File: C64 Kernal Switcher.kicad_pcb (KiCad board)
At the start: 2 copper layers, 8 parts, among them J1 LED, J2 Signals, U1 2364, U2 28C256

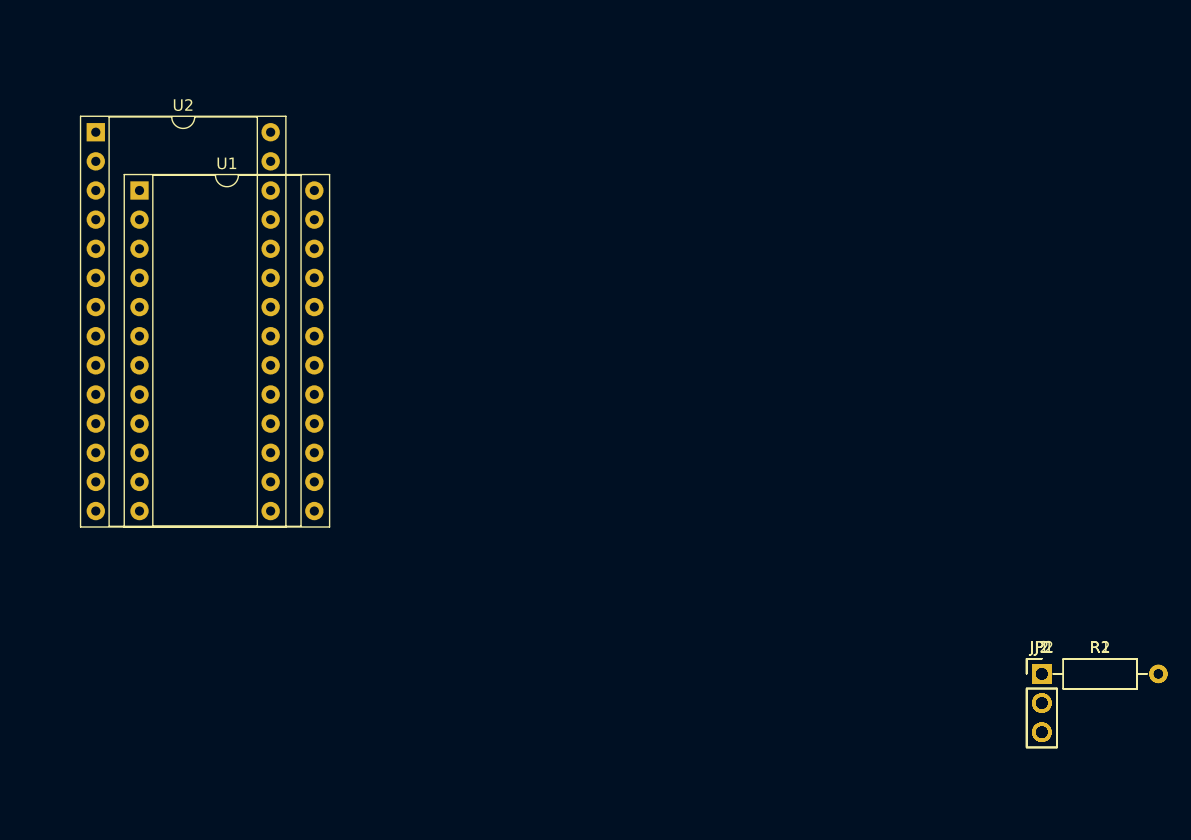
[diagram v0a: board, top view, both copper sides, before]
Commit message: PCB layed out, need measuring
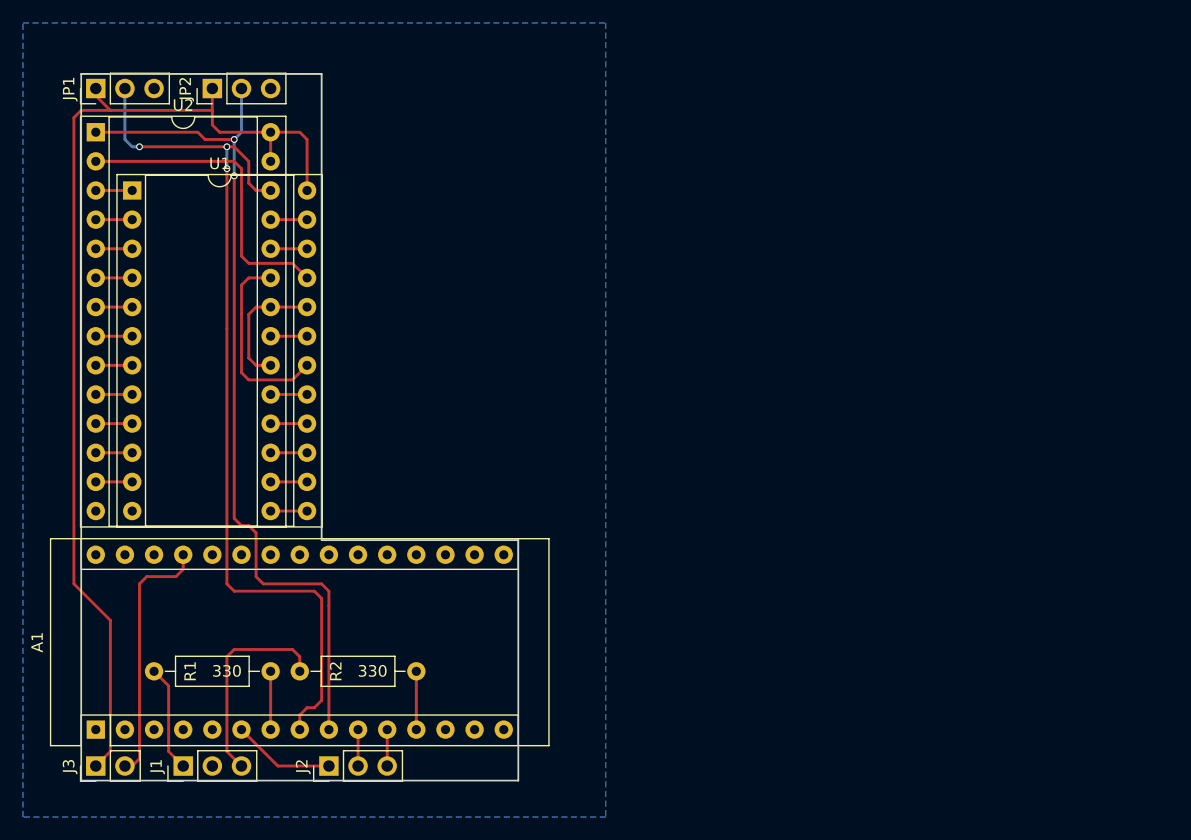
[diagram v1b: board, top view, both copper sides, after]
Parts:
- added A1: Arduino_Nano_v3.x, Modules:Arduino_Nano, F.Cu at (66.0, 109.9)
- added J3: Power, Pin_Headers:Pin_Header_Straight_1x02_Pitch2.54mm, F.Cu at (66.0, 113.0)
- moved JP1 97.0 mm to (66.0, 54.0), turned to 90 degrees
- moved JP2 88.5 mm to (76.2, 54.0), turned to 90 degrees
- moved R1 77.4 mm to (71.1, 104.8)
- moved J1 75.3 mm to (73.7, 113.0), turned to 90 degrees
- moved R2 64.7 mm to (83.8, 104.8)
- moved J2 62.7 mm to (86.4, 113.0), turned to 90 degrees
- moved U1 0.63 mm to (69.2, 62.9)
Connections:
- J2 pad 1: (no net) -> ESXROM
- J2 pad 2: (no net) -> RESET
- J2 pad 3: (no net) -> RESTORE
- R1 pad 2: (no net) -> LED1
- R2 pad 2: (no net) -> LED2
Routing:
- net VCC: track 0.00 -> 92.1 mm
- net A13: track 0.00 -> 79.6 mm, vias 0 -> 3
- net A14: track 0.00 -> 75.2 mm, vias 0 -> 2
- net /A12: track 0.00 -> 27.1 mm
- net Net-(A1-Pad27): track 0.00 -> 22.4 mm
- net Net-(J1-Pad3): track 0.00 -> 18.2 mm
- net /A11: track 0.00 -> 16.9 mm
- net /CS: track 0.00 -> 11.3 mm
- net Net-(J1-Pad1): track 0.00 -> 9.31 mm
- net ESXROM: track 0.00 -> 8.94 mm
- net LED2: track 0.00 -> 5.08 mm
- net LED1: track 0.00 -> 5.08 mm
- net RESTORE: track 0.00 -> 3.81 mm
- net RESET: track 0.00 -> 3.81 mm
- net /D7: track 0.00 -> 3.17 mm
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- added copper zone on B.Cu, net GND
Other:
- board outline added: 38.1 x 61.6 mm

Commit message: Layout redone
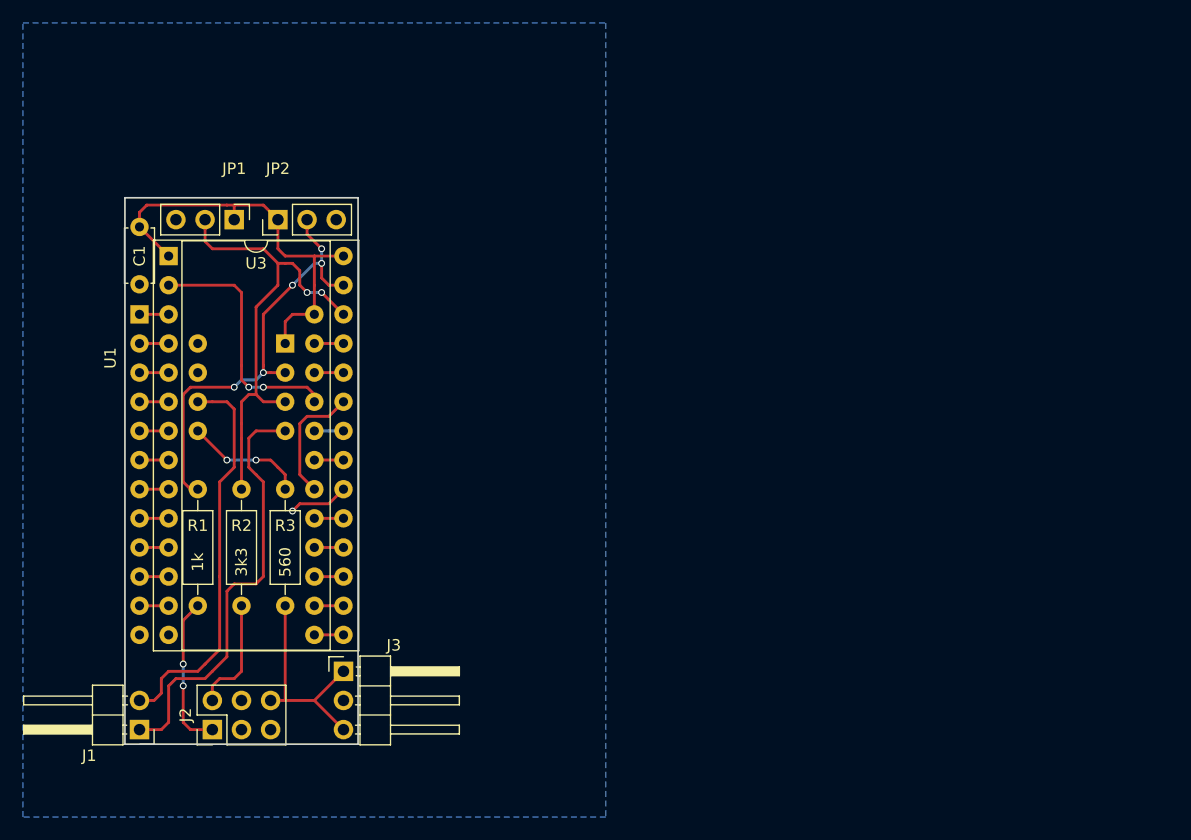
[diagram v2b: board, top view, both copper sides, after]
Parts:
- removed A1: Arduino_Nano_v3.x, Modules:Arduino_Nano
- added C1: 100nF, Capacitors_THT:C_Disc_D4.7mm_W2.5mm_P5.00mm, F.Cu at (69.8, 66.0)
- added R3: 560, Resistors_THT:R_Axial_DIN0207_L6.3mm_D2.5mm_P10.16mm_Horizontal, F.Cu at (82.5, 99.1)
- added U3: 27C256, Housings_DIP:DIP-28_W15.24mm_Socket, F.Cu at (72.4, 68.6)
- J1: value LED -> Signals; footprint Pin_Headers:Pin_Header_Straight_1x03_Pitch2.54mm -> Pin_Headers:Pin_Header_Angled_1x02_Pitch2.54mm
- J2: value Signals -> RGB; footprint Pin_Headers:Pin_Header_Straight_1x03_Pitch2.54mm -> Pin_Headers:Pin_Header_Straight_2x03_Pitch2.54mm
- J3: value Power -> LED; footprint Pin_Headers:Pin_Header_Straight_1x02_Pitch2.54mm -> Pin_Headers:Pin_Header_Angled_1x03_Pitch2.54mm
- R1: value 330 -> 1k
- R2: value 330 -> 3k3
- U1: footprint Housings_DIP:DIP-24_W15.24mm_Socket -> 2364:DIP-24_W15.24mm_Socket
- U2: value 28C256 -> PIC12F629-I/MS; footprint Housings_DIP:DIP-28_W15.24mm_Socket -> Housings_DIP:DIP-8_W7.62mm_Socket; moved to B.Cu
- moved U2 24.7 mm to (82.5, 76.2), turned to 180 degrees
- moved J3 23.1 mm to (87.6, 104.8), turned to 0 degrees
- moved JP1 16.6 mm to (78.1, 65.4), turned to 270 degrees
- moved JP2 12.8 mm to (81.9, 65.4)
- moved U1 10.8 mm to (69.8, 73.7)
- moved J2 10.6 mm to (76.2, 109.9)
- moved R2 7.65 mm to (78.7, 99.1), turned to 90 degrees
- moved R1 6.87 mm to (74.9, 99.1), turned to 90 degrees
- moved J1 4.96 mm to (69.8, 109.9), turned to 180 degrees
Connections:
- J1 pad 1: Net-(J1-Pad1) -> ~RESTORE
- J1 pad 2: GND -> ~RESET
- J2 pad 1: ESXROM -> BLUE
- J2 pad 2: RESET -> GREEN
- J2 pad 3: RESTORE -> GND
- J3 pad 1: VCC -> RED
- J3 pad 2: Net-(A1-Pad27) -> GND
- R1 pad 1: Net-(J1-Pad1) -> BLUE
- R1 pad 2: LED1 -> A14
- R2 pad 1: Net-(J1-Pad3) -> GREEN
- R2 pad 2: LED2 -> A13
- U2 pad 1: A14 -> VCC
- U2 pad 2: /A12 -> A14
- U2 pad 3: /A7 -> A13
- U2 pad 4: /A6 -> ~RESTORE
- U2 pad 5: /A5 -> Net-(R3-Pad2)
- U2 pad 6: /A4 -> ~RESET
- U2 pad 7: /A3 -> (no net)
- U2 pad 8: /A2 -> GND
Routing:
- net VCC: track 92.1 -> 37.9 mm
- net A13: track 79.6 -> 41.5 mm, vias 3 -> 2
- net ~RESTORE: track 0.00 -> 37.6 mm
- net A14: track 75.2 -> 38.6 mm, vias 2 -> 5
- net ~RESET: track 0.00 -> 34.5 mm
- net Net-(A1-Pad27): track 22.4 -> 0.00 mm
- net RED: track 0.00 -> 19.2 mm
- net Net-(J1-Pad3): track 18.2 -> 0.00 mm
- net BLUE: track 0.00 -> 13.5 mm, vias 0 -> 2
- net Net-(R3-Pad2): track 0.00 -> 10.5 mm, vias 0 -> 2
- net GREEN: track 0.00 -> 10.1 mm
- net Net-(J1-Pad1): track 9.31 -> 0.00 mm
- net ESXROM: track 8.94 -> 0.00 mm
- net /CS: track 11.3 -> 3.17 mm
- net /A11: track 16.9 -> 10.8 mm
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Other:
- board size 38.1 x 61.6 mm -> 20.3 x 47.6 mm
